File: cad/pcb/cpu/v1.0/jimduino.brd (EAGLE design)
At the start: 38 x 31 mm, 61 parts, among them CN1 SM02B-SRSS-TB, P1 DF12-32-DP, P2 DF12-32-DP, P3 MICROUSB, Q1 FDN360P, Q2 FDN360P, SW1 SWITCH-MOMENTARY-2SMD-REDUNDA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, U1 STM32F415R, U2 MCP1703, U3 MCP73831, U4 LTC2954-2, Y1 8Y-16.000MAAV-T, Y2 32.768kHz

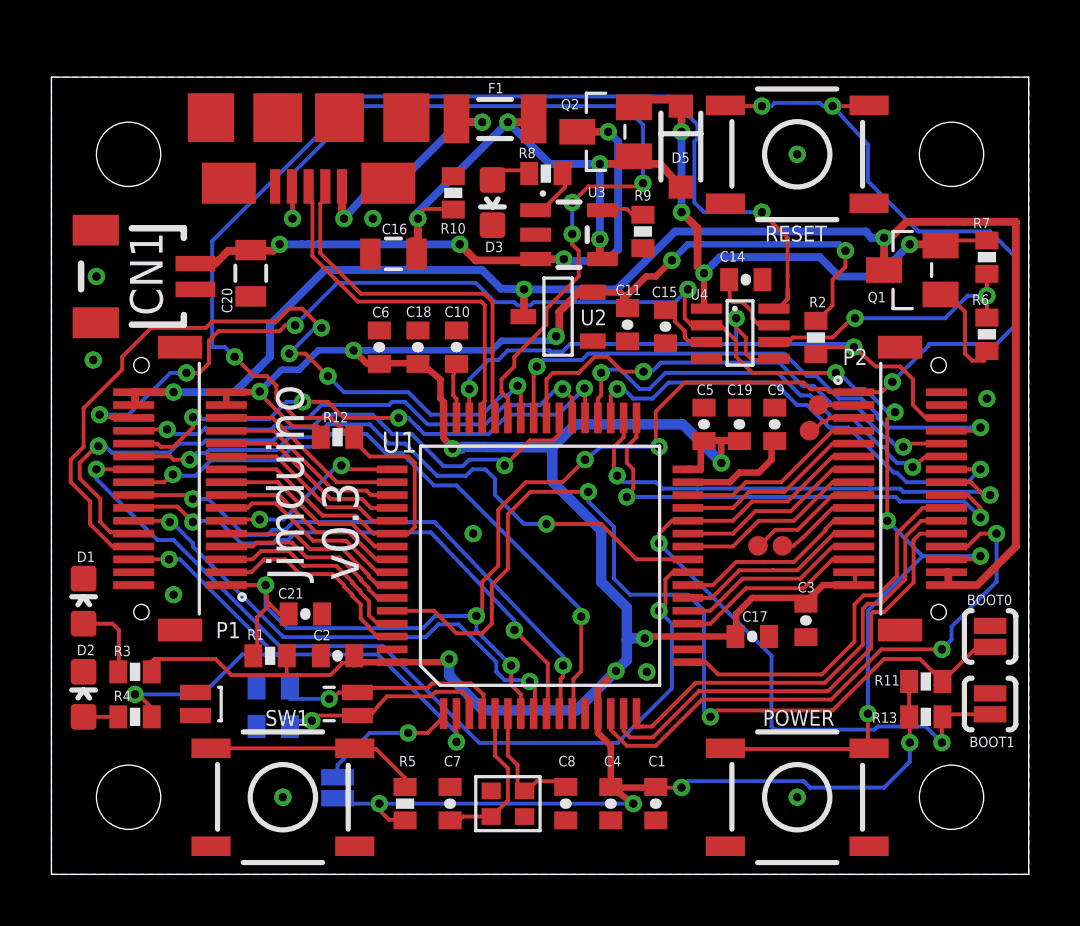
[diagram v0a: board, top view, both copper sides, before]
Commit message: Release Candidate 2
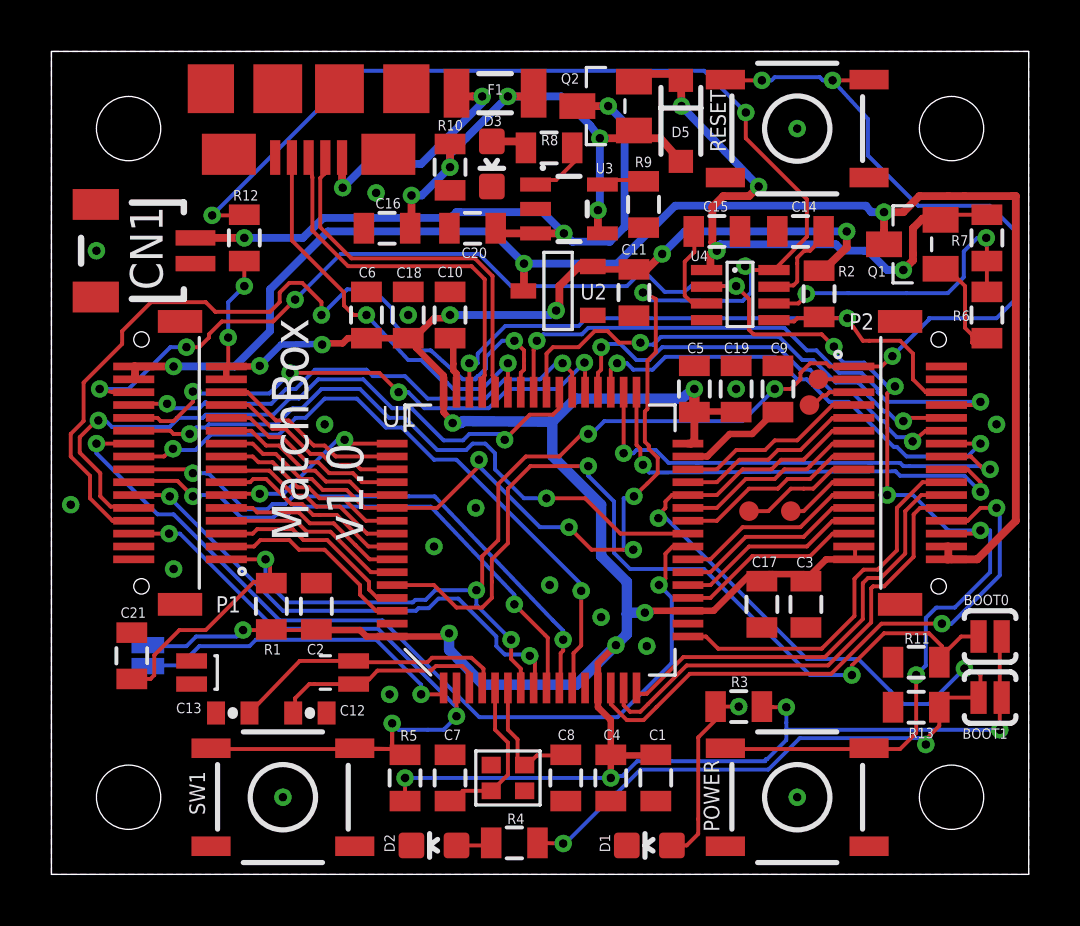
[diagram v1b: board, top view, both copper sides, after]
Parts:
- BOOT0, BOOT1: value JUMPER-PAD-2-NC_BY_PASTE -> JUMPER-PAD-2-NOYES_SILK; device SparkFun-Passives:PAD-JUMPER-2-NC_BY_PASTE_YES_SILK -> SparkFun-Passives:PAD-JUMPER-2-NO_YES_SILK
- C1, C10, C11, C14, C15, C17, C18, C19, C2, C21, C3, C4, C5, C6, C9: device SparkFun-Capacitors:0402-CAP -> SparkFun-Capacitors:0805
- C12, C13: value 20pF -> 4pF
- C7, C8: value 20pF -> 4pF; device SparkFun-Capacitors:0402-CAP -> SparkFun-Capacitors:0805
- D2: value PC13 -> BOOT1
- R1, R10, R11, R12, R13, R2, R3, R4, R5, R6, R7, R8, R9: device SparkFun-Passives:0402-RES -> SparkFun-Passives:0805
- Y1: value 8Y-16.000MAAV-T -> 16MHz(9pF)
- Y2: value 32.768kHz -> 32.768kHz (9pF)
- moved D1 24.0 mm to (23.2, 1.12), turned to 90 degrees
- moved R3 23.5 mm to (26.7, 6.53)
- moved R4 15.5 mm to (18.0, 1.23)
- moved D2 14.8 mm to (14.9, 1.12), turned to 90 degrees
- moved BKUP 8.98 mm to (3.75, 8.50), turned to 90 degrees
- moved C20 8.80 mm to (16.4, 25.1), turned to 180 degrees
- moved R12 8.56 mm to (7.50, 24.8), turned to 90 degrees
- moved C21 6.94 mm to (3.12, 8.50), turned to 90 degrees
- moved C15 4.21 mm to (25.9, 25.0), turned to 0 degrees
- moved C14 2.83 mm to (29.1, 25.0), turned to 180 degrees
- moved C2 2.09 mm to (10.3, 10.4), turned to 90 degrees
- moved R1 1.93 mm to (8.55, 10.4), turned to 270 degrees
- moved C13 1.85 mm to (7.05, 6.28), flipped to the top, turned to 180 degrees
- moved R2 1.70 mm to (29.9, 22.6)
- moved C12 1.52 mm to (10.1, 6.28), flipped to the top
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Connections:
- removed net PC14: R5.1, SW1.1, SW1.2
- net GND: now also R11.2, R13.2; no longer BOOT0.2, BOOT1.2
- net PB2: now also R4.2
- net PC13: now also R5.1, SW1.1, SW1.2; no longer R4.2
- net VCC_3V3: now also BOOT0.2, BOOT1.2; no longer R11.2, R13.2
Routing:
- net PB2: track 28.0 -> 47.0 mm, vias 2 -> 4
- net PA10: track 33.7 -> 16.0 mm, vias 4 -> 2
- net PD2: track 58.1 -> 70.9 mm, vias 2 -> 8
- net PC14: track 8.37 -> 0.00 mm
- net VCC_BKUP: track 5.50 -> 13.6 mm
- net VCC_3V3: track 142.3 -> 135.2 mm, vias 14 -> 18
- net PC13: track 24.5 -> 31.2 mm
- net VBAT: track 23.7 -> 28.5 mm, vias 4 -> 3
- net PWR_ON: track 62.7 -> 67.0 mm
- net N$5: track 3.13 -> 7.34 mm, vias 0 -> 1
- net RESET#: track 70.0 -> 73.3 mm
- net N$3: track 2.55 -> 5.33 mm
- net BOOT0: track 37.8 -> 35.2 mm
- net PA13: track 28.0 -> 25.6 mm, vias 3 -> 2
- net N$8: track 10.7 -> 12.8 mm
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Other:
- board size 38 x 31 mm -> 38 x 32 mm
- board text added: "MatchBox v1.0"
- board text removed: "Jimduino v0.3"
